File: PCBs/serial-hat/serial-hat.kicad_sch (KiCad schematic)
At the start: 11 parts, among them CN1 Modem port, CN2 Printer port, J1 Conn_01x02_Pin, J7 Rpi headers, U1 PC817C-S, U2 MAX3232

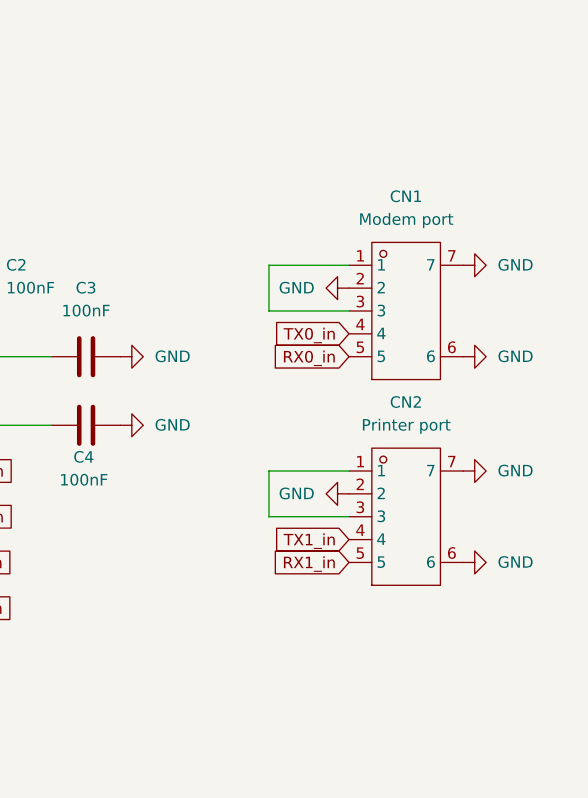
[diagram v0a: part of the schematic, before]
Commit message: Update to new lib
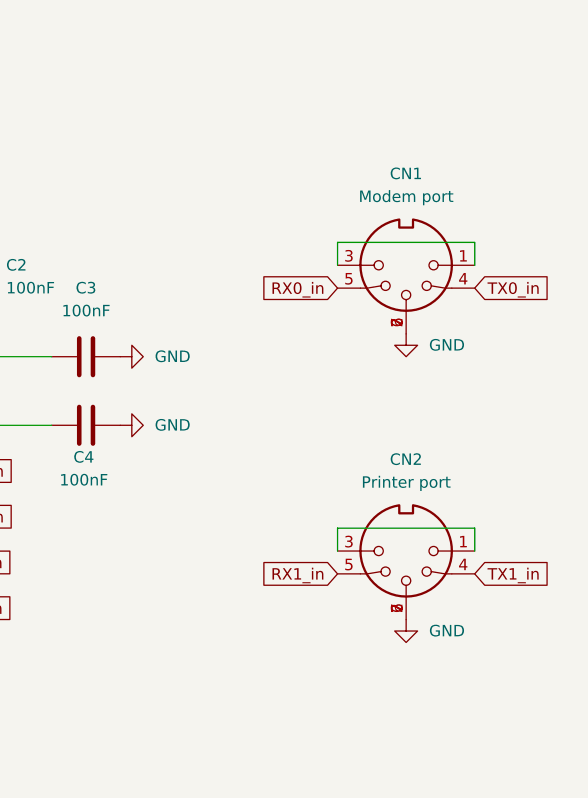
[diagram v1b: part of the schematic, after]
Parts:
- CN1, CN2: footprint DIN5:CONN-TH_DIN-504-M10 -> Colins-Kicad:DIN-5-M C2939346; symbol DIN:DIN-504 -> Colins-Kicad:DIN-5_180degree
- U1: footprint Package_SO:SOP-4_3.8x4.1mm_P2.54mm -> Colins-Kicad:PC817C-S C3008369
